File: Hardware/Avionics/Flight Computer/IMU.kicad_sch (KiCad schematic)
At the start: 4 parts, among them U1 BNO055

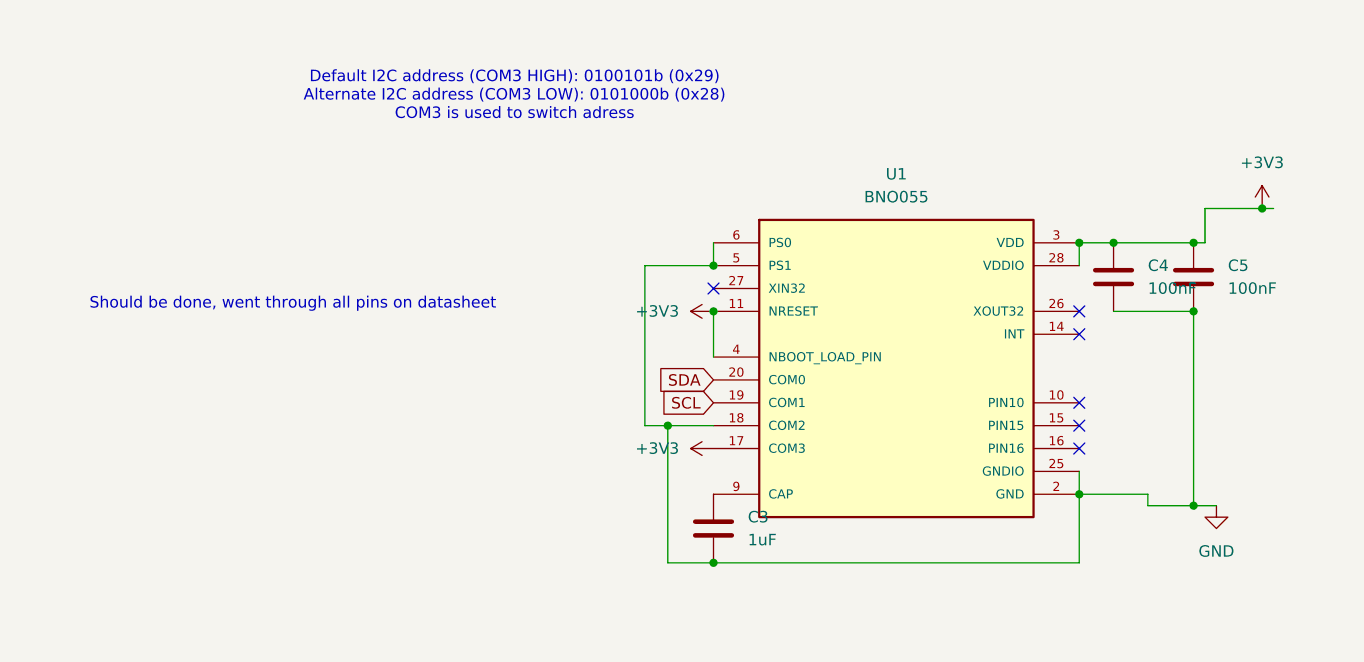
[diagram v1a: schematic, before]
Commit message: updated FC
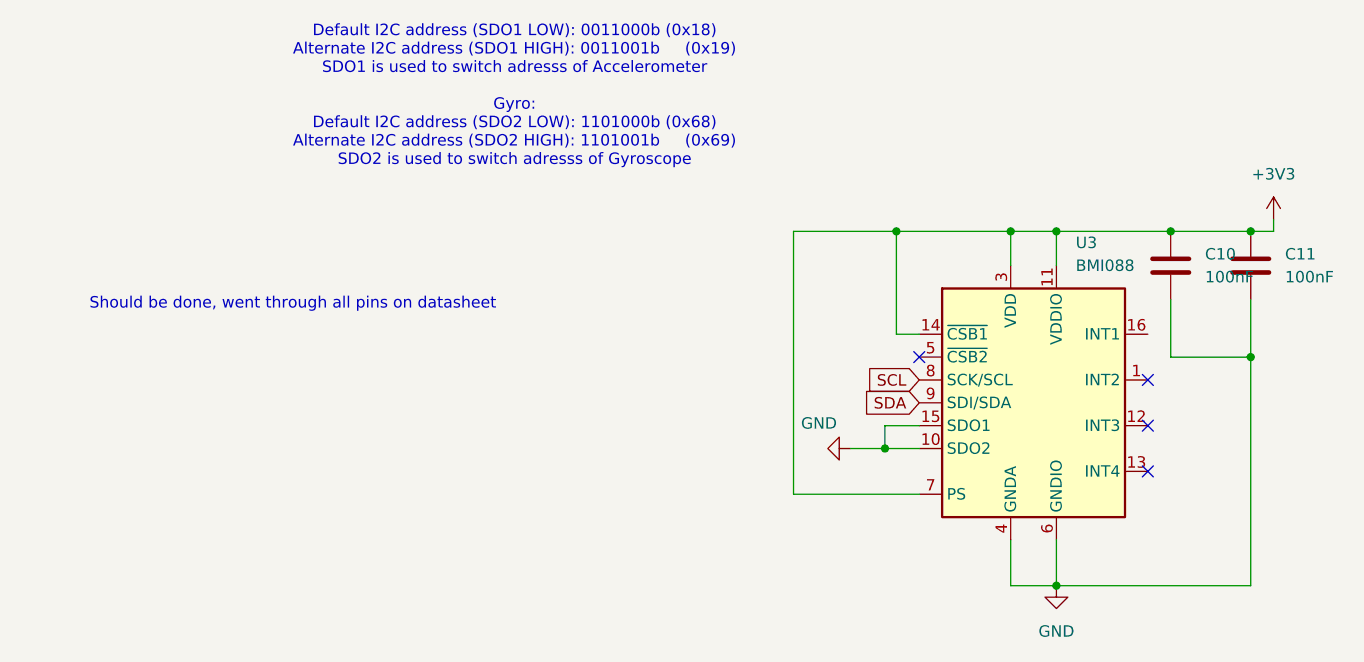
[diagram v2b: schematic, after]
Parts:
- removed C3: 1uF, Capacitor_SMD:C_0805_2012Metric, symbol Device:C
- removed C4, C5: 100nF, Capacitor_SMD:C_0805_2012Metric, symbol Device:C
- removed U1: BNO055, Package_LGA:LGA-28_5.2x3.8mm_P0.5mm, symbol SRAD:BNO055
- added C10, C11: 100nF, Capacitor_SMD:C_0805_2012Metric, symbol Device:C
- added U3: BMI088, Package_LGA:Bosch_LGA-16_4.5x3mm_P0.5mm_LayoutBorder7x1y_ClockwisePinNumbering, symbol Sensor_Motion:BMI088
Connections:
- net +3V3: now also C10.1, C11.1, U3.11 (VDDIO), U3.14 (~{CSB1}), U3.3 (VDD), U3.7 (PS)
- net GND: now also C10.2, C11.2, U3.10 (SDO2), U3.15 (SDO1), U3.2 (GNDA), U3.4 (GNDA), U3.6 (GNDIO)
- net SCL: now also U3.8 (SCK/SCL)
- net SDA: now also U3.9 (SDI/SDA)
- no-connect marks 6 -> 4
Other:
- note added: "Default I2C address (SDO1 LOW): 0011000b (0x18) Alternate I2C address (SDO1 HIGH): 0011001b (0x19) SDO1 is used to switch adresss of Accelerometer Gyro: Default I2C address (SDO2 LOW): 1101000b (0x68) Alternate I2C address (SDO2 HIGH): 1101001b (0x69) SDO2 is used to switch adresss of Gyroscope"
- note removed: "Default I2C address (COM3 HIGH): 0100101b (0x29) Alternate I2C address (COM3 LOW): 0101000b (0x28) COM3 is used to switch adress"
